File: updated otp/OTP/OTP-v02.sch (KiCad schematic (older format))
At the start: 32 parts, among them J1 FPC24, J2 Conn_01x06_Female, Q1 2N7000, Q2 PN2222A, SW1 Switch_SW_Push, U1 ATmega328P-AU, U2 DS3231M

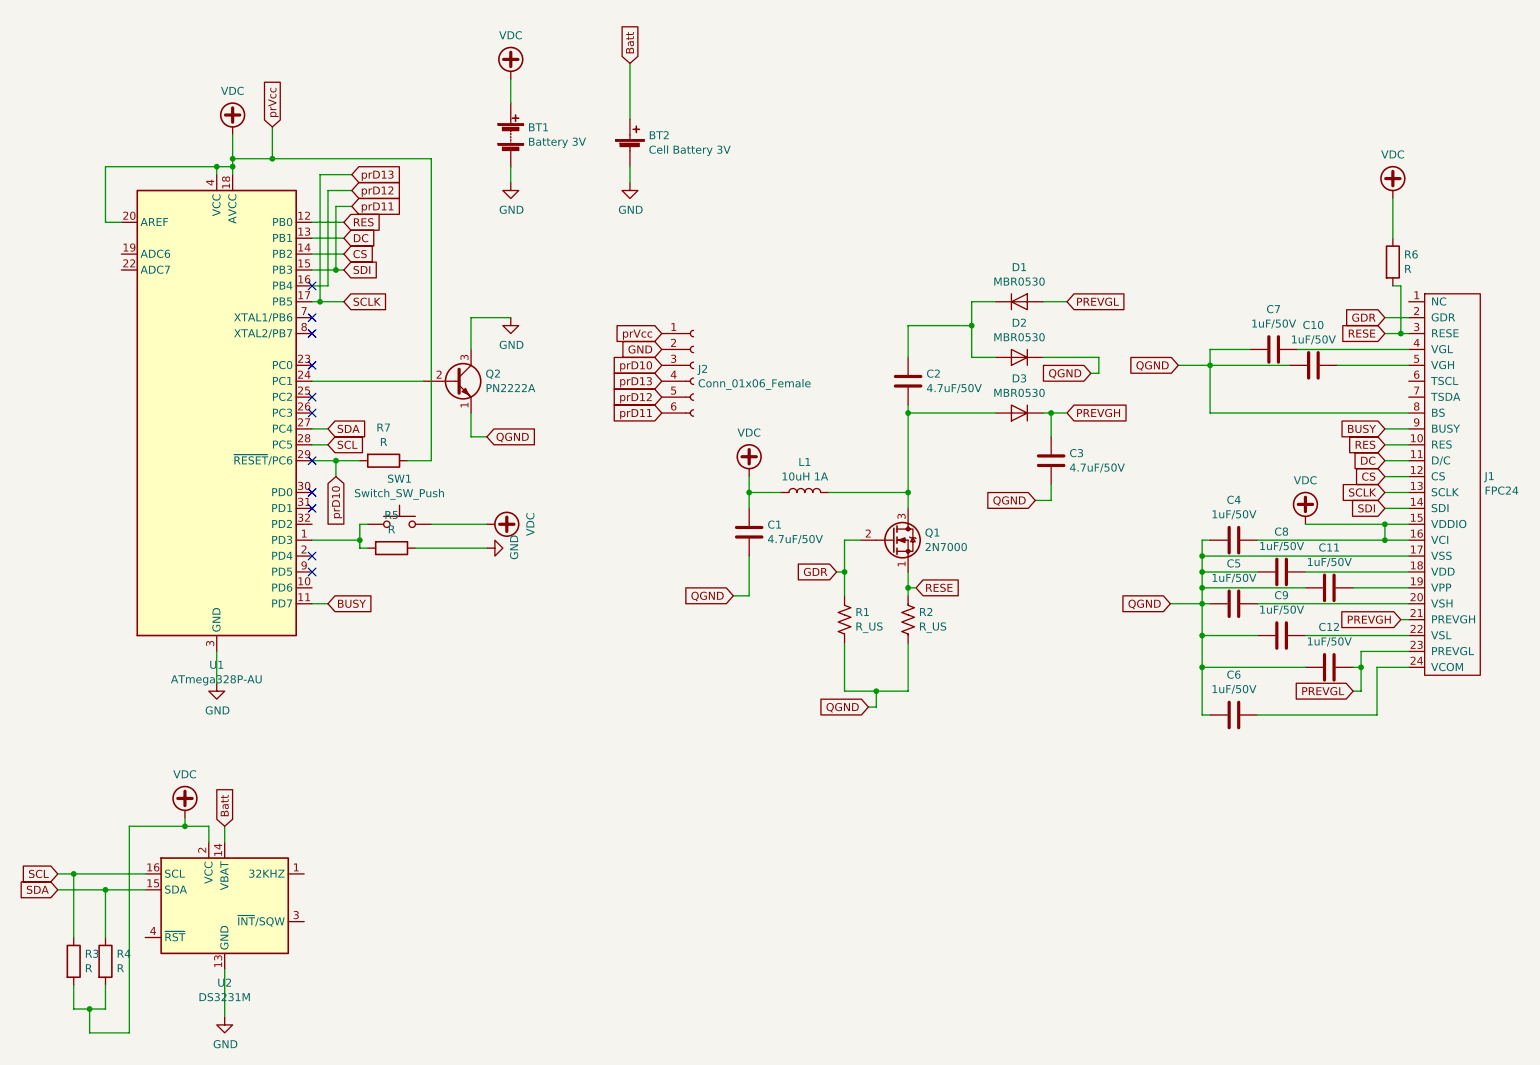
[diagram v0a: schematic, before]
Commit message: First Commit
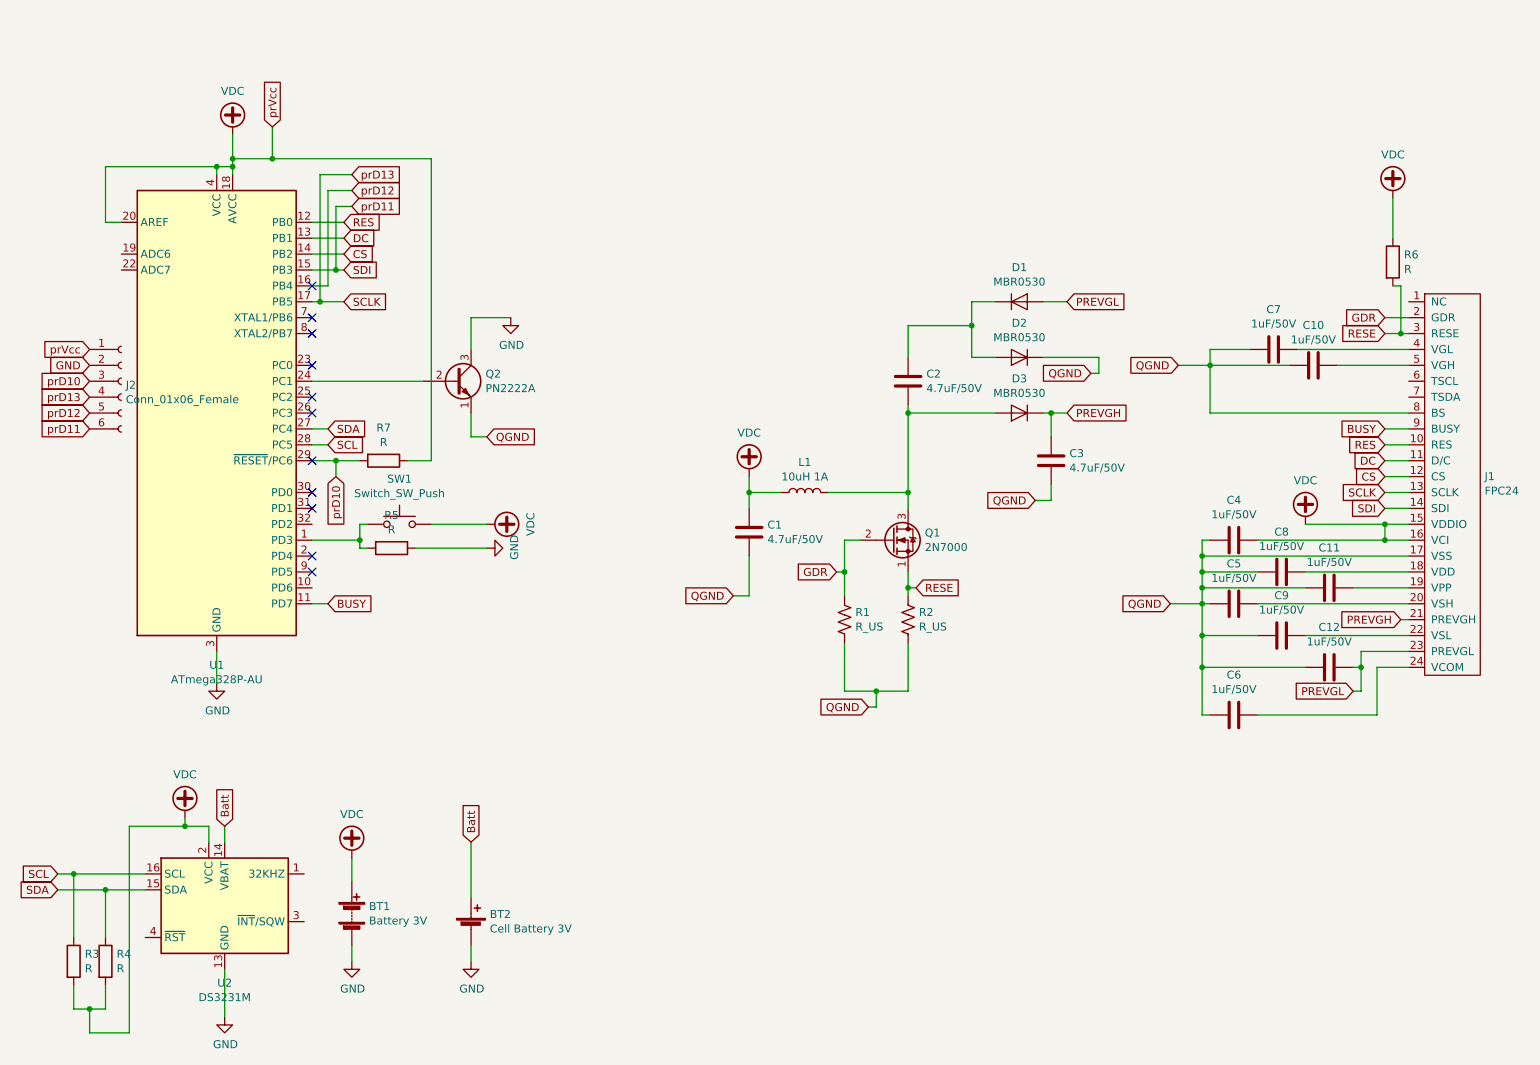
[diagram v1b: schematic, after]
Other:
- moved on the sheet: BT1, BT2, J2
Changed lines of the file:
@@
 $EndDescr
-$Comp
-L OTP-v02-rescue:FPC24-otp J1
-U 1 1 5C7151EB
-P 9700 3350
-F 0 "J1" H 10077 3301 50  0000 L CNN
-F 1 "FPC24" H 10077 3210 50  0000 L CNN
-F 2 "otp:FPC24" H 9700 2500 50  0001 C CNN
-F 3 "" H 9700 2500 50  0001 C CNN
-	1    9700 3350
-	1    0    0    -1
-$EndComp
 $Comp
 L Device:C C7
@@
 Connection ~ 8300 4000
 Wire Wire Line
-	8300 4000 8300 3900
-Wire Wire Line
 	8950 4100 8300 4100
 Connection ~ 8300 4100
 Wire Wire Line
 	8300 4100 8300 4000
-Wire Wire Line
-	9600 3900 8300 3900
-Connection ~ 8300 3900
-Wire Wire Line
-	8300 3900 8300 3800
 Wire Wire Line
 	8650 4400 8300 4400
@@
 L Device:Battery_Cell BT2
 U 1 1 5C7C1C30
-P 4700 1350
-F 0 "BT2" H 4818 1446 50  0000 L CNN
-F 1 "Cell Battery 3V" H 4818 1355 50  0000 L CNN
-F 2 "otp:Cell Battery SMD" V 4700 1410 50  0001 C CNN
-F 3 "~" V 4700 1410 50  0001 C CNN
-	1    4700 1350
-	1    0    0    -1
-$EndComp
-Wire Wire Line
-	4700 800  4700 1150
+P 3700 6250
+F 0 "BT2" H 3818 6346 50  0000 L CNN
+F 1 "Cell Battery 3V" H 3818 6255 50  0000 L CNN
+F 2 "otp:Cell Battery SMD" V 3700 6310 50  0001 C CNN
+F 3 "~" V 3700 6310 50  0001 C CNN
+	1    3700 6250
+	1    0    0    -1
+$EndComp
+Wire Wire Line
+	3700 5700 3700 6050
 $Comp
 L power:GND #PWR011
 U 1 1 5C7C6F65
-P 4700 1550
-F 0 "#PWR011" H 4700 1300 50  0001 C CNN
-F 1 "GND" H 4705 1377 50  0000 C CNN
-F 2 "" H 4700 1550 50  0001 C CNN
-F 3 "" H 4700 1550 50  0001 C CNN
-	1    4700 1550
-	1    0    0    -1
-$EndComp
-Wire Wire Line
-	4700 1550 4700 1450
+P 3700 6450
+F 0 "#PWR011" H 3700 6200 50  0001 C CNN
+F 1 "GND" H 3705 6277 50  0000 C CNN
+F 2 "" H 3700 6450 50  0001 C CNN
+F 3 "" H 3700 6450 50  0001 C CNN
+	1    3700 6450
+	1    0    0    -1
+$EndComp
+Wire Wire Line
+	3700 6450 3700 6350
 $Comp
 L Device:Battery BT1
 U 1 1 5C7CB3D8
-P 3950 1250
-F 0 "BT1" H 4058 1296 50  0000 L CNN
-F 1 "Battery 3V" H 4058 1205 50  0000 L CNN
-F 2 "otp:Battery_pack_connector" V 3950 1310 50  0001 C CNN
-F 3 "~" V 3950 1310 50  0001 C CNN
-	1    3950 1250
+P 2950 6150
+F 0 "BT1" H 3058 6196 50  0000 L CNN
+F 1 "Battery 3V" H 3058 6105 50  0000 L CNN
+F 2 "otp:Battery_pack_connector" V 2950 6210 50  0001 C CNN
+F 3 "~" V 2950 6210 50  0001 C CNN
+	1    2950 6150
 	1    0    0    -1
 $EndComp
@@
 L power:VDC #PWR08
 U 1 1 5C7CB490
-P 3950 900
-F 0 "#PWR08" H 3950 800 50  0001 C CNN
-F 1 "VDC" H 3950 1175 50  0000 C CNN
-F 2 "" H 3950 900 50  0001 C CNN
-F 3 "" H 3950 900 50  0001 C CNN
-	1    3950 900
-	1    0    0    -1
-$EndComp
-Wire Wire Line
-	3950 900  3950 1050
+P 2950 5800
+F 0 "#PWR08" H 2950 5700 50  0001 C CNN
+F 1 "VDC" H 2950 6075 50  0000 C CNN
+F 2 "" H 2950 5800 50  0001 C CNN
+F 3 "" H 2950 5800 50  0001 C CNN
+	1    2950 5800
+	1    0    0    -1
+$EndComp
+Wire Wire Line
+	2950 5800 2950 5950
 $Comp
 L power:GND #PWR09
 U 1 1 5C7D3CE3
-P 3950 1550
-F 0 "#PWR09" H 3950 1300 50  0001 C CNN
-F 1 "GND" H 3955 1377 50  0000 C CNN
-F 2 "" H 3950 1550 50  0001 C CNN
-F 3 "" H 3950 1550 50  0001 C CNN
-	1    3950 1550
-	1    0    0    -1
-$EndComp
-Wire Wire Line
-	3950 1550 3950 1450
+P 2950 6450
+F 0 "#PWR09" H 2950 6200 50  0001 C CNN
+F 1 "GND" H 2955 6277 50  0000 C CNN
+F 2 "" H 2950 6450 50  0001 C CNN
+F 3 "" H 2950 6450 50  0001 C CNN
+	1    2950 6450
+	1    0    0    -1
+$EndComp
+Wire Wire Line
+	2950 6450 2950 6350
 NoConn ~ 2700 2200
 NoConn ~ 2700 2400
@@
 Wire Wire Line
 	9450 3400 9600 3400
-Text GLabel 4700 800  1    50   Input ~ 0
+Text GLabel 3700 5700 1    50   Input ~ 0
 Batt
 Text GLabel 2150 5600 1    50   Input ~ 0
@@
 L Connector:Conn_01x06_Female J2
 U 1 1 5CDD3003
-P 5100 2700
-F 0 "J2" H 5128 2676 50  0000 L CNN
-F 1 "Conn_01x06_Female" H 5128 2585 50  0000 L CNN
-F 2 "otp:programmer06" H 5100 2700 50  0001 C CNN
-F 3 "~" H 5100 2700 50  0001 C CNN
-	1    5100 2700
-	1    0    0    -1
-$EndComp
-Text GLabel 4900 2500 0    50   Input ~ 0
+P 1500 2800
+F 0 "J2" H 1528 2776 50  0000 L CNN
+F 1 "Conn_01x06_Female" H 1528 2685 50  0000 L CNN
+F 2 "otp:programmer06" H 1500 2800 50  0001 C CNN
+F 3 "~" H 1500 2800 50  0001 C CNN
+	1    1500 2800
+	1    0    0    -1
+$EndComp
+Text GLabel 1300 2600 0    50   Input ~ 0
 prVcc
-Text GLabel 4900 2600 0    50   Input ~ 0
+Text GLabel 1300 2700 0    50   Input ~ 0
 GND
-Text GLabel 4900 2700 0    50   Input ~ 0
+Text GLabel 1300 2800 0    50   Input ~ 0
 prD10
-Text GLabel 4900 3000 0    50   Input ~ 0
+Text GLabel 1300 3100 0    50   Input ~ 0
 prD11
-Text GLabel 4900 2900 0    50   Input ~ 0
+Text GLabel 1300 3000 0    50   Input ~ 0
 prD12
-Text GLabel 4900 2800 0    50   Input ~ 0
+Text GLabel 1300 2900 0    50   Input ~ 0
 prD13
 Wire Wire Line
@@
 Text GLabel 2850 3400 3    50   Input ~ 0
 prD10
+$Comp
+L OTP-v02-rescue:FPC24-otp J1
+U 1 1 5C7151EB
+P 9700 3350
+F 0 "J1" H 10077 3301 50  0000 L CNN
+F 1 "FPC24" H 10077 3210 50  0000 L CNN
+F 2 "otp:FPC24" H 9700 2500 50  0001 C CNN
+F 3 "" H 9700 2500 50  0001 C CNN
+	1    9700 3350
+	1    0    0    -1
+$EndComp
+Wire Wire Line
+	8300 4000 8300 3900
+Wire Wire Line
+	8300 3900 8300 3800
+Connection ~ 8300 3900
+Wire Wire Line
+	9600 3900 8300 3900
 $EndSCHEMATC
